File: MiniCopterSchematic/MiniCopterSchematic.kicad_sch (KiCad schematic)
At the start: 19 parts, among them J1 MPU6050_IMU, M1 MOTOR_DC, M2 MOTOR_DC, M3 MOTOR_DC, M4 MOTOR_DC, Q1 IRF540N, Q2 IRF540N, Q3 IRF540N, Q4 IRF540N

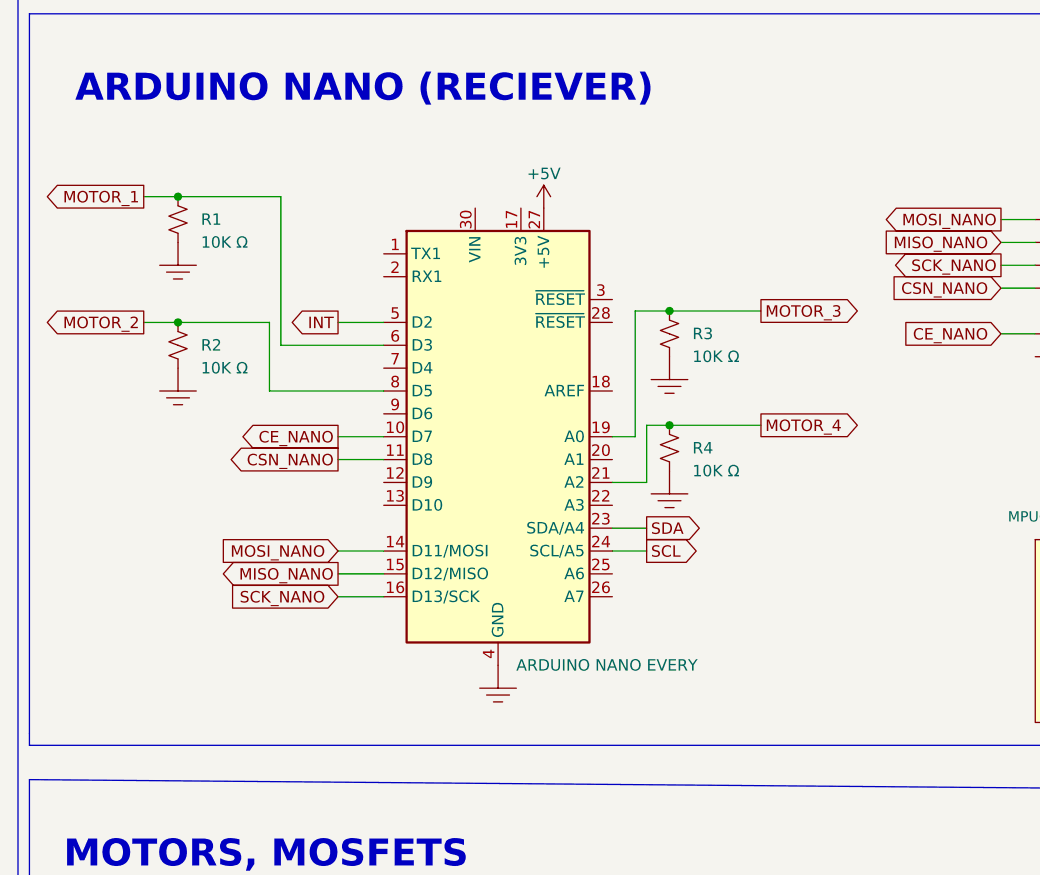
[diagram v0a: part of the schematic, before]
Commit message: Updated schematic
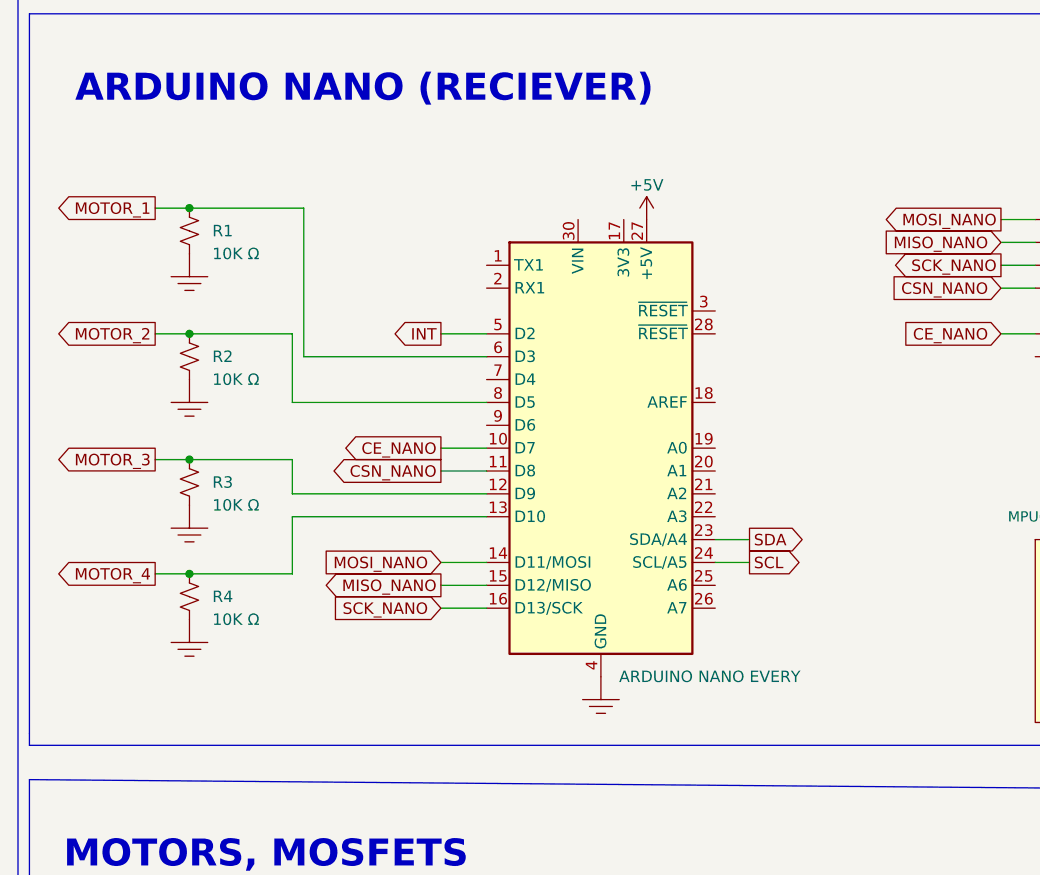
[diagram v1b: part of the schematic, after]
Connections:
- net MOTOR_3: now also A1.12 (D9); no longer A1.19 (A0)
- net MOTOR_4: now also A1.13 (D10); no longer A1.21 (A2)
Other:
- moved on the sheet: R1, R2, R3, R4
